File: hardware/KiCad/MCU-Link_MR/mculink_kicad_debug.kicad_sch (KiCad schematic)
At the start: 43 parts, among them J1 Pixhawk Debug Full (1x10 JST-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, J2 Pixhawk_Debug_Mini (1x06 JST-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, J6 Conn_02x05_Odd_Even, J8 DCD-LZ_Debug (1x07 JST-GHS), SW2 KMR221GLFS, U3 74LVC2T45DC, U4 SN74LVC1T45GW, U5 SN74LVC1T45GW, U6 MCP6001-OT, U7 SN74LVC1T45GW

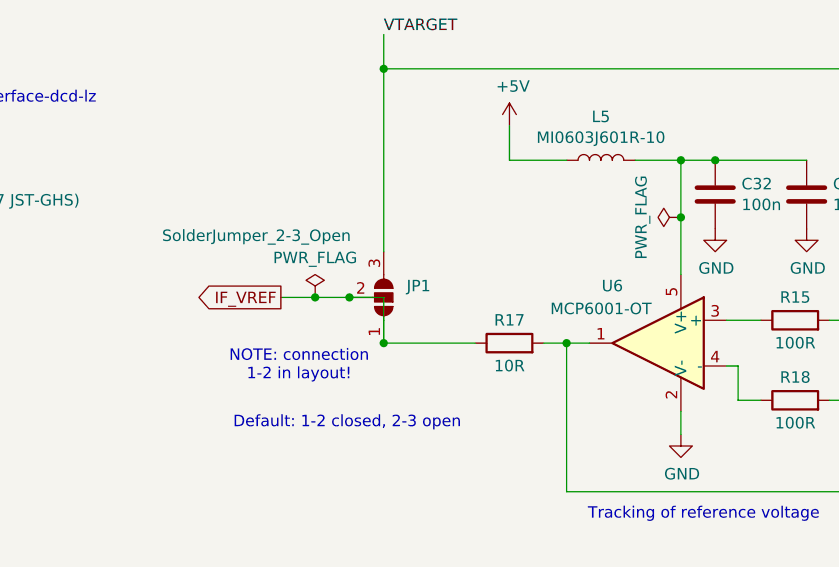
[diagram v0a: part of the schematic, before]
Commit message: cleanup
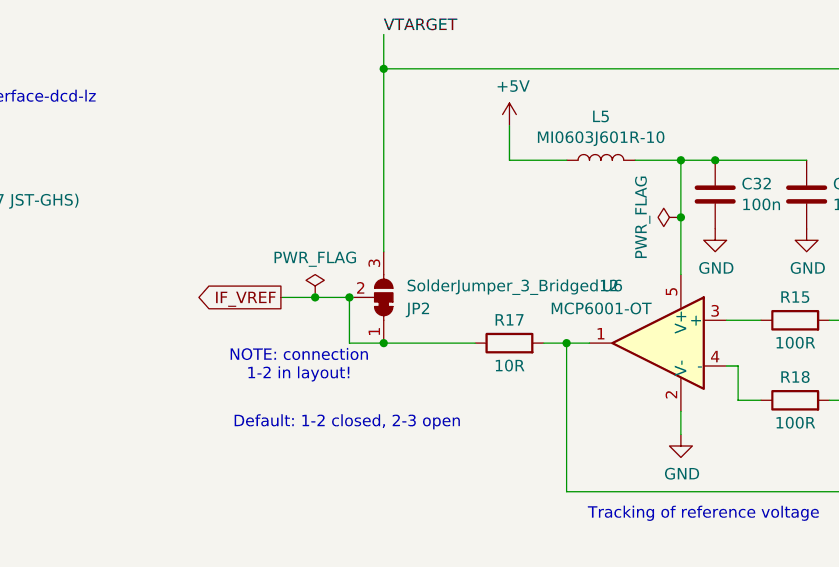
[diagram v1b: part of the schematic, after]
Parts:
- removed JP1: SolderJumper_2-3_Open, McuOnEclipse:SolderJumper-3_P1.3mm_Open_RoundedPad1.0x1.5mm, symbol Jumper:SolderJumper_3_Open
- added JP2: SolderJumper_3_Bridged12, McuOnEclipse:SolderJumper-3_P1.3mm_Open_RoundedPad1.0x1.5mm, symbol Jumper:SolderJumper_3_Bridged12
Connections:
- net IF_VREF: now also JP2.1 (A), JP2.2 (C)
- net VTARGET: now also JP2.3 (B)
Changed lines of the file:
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@@
 	)
 	(junction
-		(at 203.2 134.62)
-		(diameter 0)
-		(color 0 0 0 0)
-	)
-	(junction
 		(at 63.5 20.32)
 		(diameter 0)
@@
 	)
 	(junction
+		(at 203.2 134.62)
+		(diameter 0)
+		(color 0 0 0 0)
+	)
+	(junction
 		(at 240.03 119.38)
 		(diameter 0)
@@
 	)
 	(junction
-		(at 207.01 139.7)
-		(diameter 0)
-		(color 0 0 0 0)
-	)
-	(junction
 		(at 227.33 139.7)
 		(diameter 0)
@@
 	)
 	(junction
+		(at 207.01 139.7)
+		(diameter 0)
+		(color 0 0 0 0)
+	)
+	(junction
 		(at 33.02 20.32)
 		(diameter 0)
@@
 	(wire
 		(pts
+			(xy 203.2 134.62) (xy 203.2 139.7)
+		)
+		(stroke
+			(width 0)
+			(type default)
+		)
+	)
+	(wire
+		(pts
 			(xy 267.97 48.26) (xy 271.78 48.26)
 		)
@@
 	(wire
 		(pts
-			(xy 207.01 134.62) (xy 203.2 134.62)
-		)
-		(stroke
-			(width 0)
-			(type default)
-		)
-	)
-	(wire
-		(pts
 			(xy 257.81 156.21) (xy 227.33 156.21)
 		)
@@
 	(wire
 		(pts
-			(xy 207.01 139.7) (xy 207.01 134.62)
-		)
-		(stroke
-			(width 0)
-			(type default)
-		)
-	)
-	(wire
-		(pts
 			(xy 96.52 179.07) (xy 96.52 180.34)
 		)
@@
 	(wire
 		(pts
+			(xy 203.2 139.7) (xy 207.01 139.7)
+		)
+		(stroke
+			(width 0)
+			(type default)
+		)
+	)
+	(wire
+		(pts
 			(xy 39.37 125.73) (xy 39.37 124.46)
 		)
@@
 	)
 	(symbol
+		(lib_id "Jumper:SolderJumper_3_Bridged12")
+		(at 207.01 134.62 270)
+		(mirror x)
+		(unit 1)
+		(exclude_from_sim no)
+		(in_bom yes)
+		(on_board yes)
+		(dnp no)
+		(fields_autoplaced yes)
+		(property "Reference" "JP2"
+			(at 209.55 135.8901 90)
+			(effects
+				(font
+					(size 1.27 1.27)
+				)
+				(justify left)
+			)
+		)
+		(property "Value" "SolderJumper_3_Bridged12"
+			(at 209.55 133.3501 90)
+			(effects
+				(font
+					(size 1.27 1.27)
+				)
+				(justify left)
+			)
+		)
+		(property "Footprint" "McuOnEclipse:SolderJumper-3_P1.3mm_Open_RoundedPad1.0x1.5mm"
+			(at 207.01 134.62 0)
+			(effects
+				(font
+					(size 1.27 1.27)
+				)
+				(hide yes)
+			)
+		)
+		(property "Datasheet" "~"
+			(at 207.01 134.62 0)
+			(effects
+				(font
+					(size 1.27 1.27)
+				)
+				(hide yes)
+			)
+		)
+		(property "Description" "3-pole Solder Jumper, pins 1+2 closed/bridged"
+			(at 207.01 134.62 0)
+			(effects
+				(font
+					(size 1.27 1.27)
+				)
+				(hide yes)
+			)
+		)
+		(pin "3"
+		)
+		(pin "2"
+		)
+		(pin "1"
+		)
+		(instances
+			(project "MCU-Link_MR"
+				(path "/5d025764-753a-4b80-8d3d-c9a8a22c9527/00000000-0000-0000-0000-0000603cff19"
+					(reference "JP2")
+					(unit 1)
+				)
+			)
+		)
+	)
+	(symbol
 		(lib_id "power:GND")
 		(at 143.51 102.87 0)
@@
 					(unit 1)
 				)
-			)
-		)
-	)
-	(symbol
-		(lib_id "Jumper:SolderJumper_3_Open")
-		(at 207.01 134.62 270)
-		(mirror x)
-		(unit 1)
-		(exclude_from_sim no)
-		(in_bom yes)
-		(on_board yes)
-		(dnp no)
-		(property "Reference" "JP1"
-			(at 209.55 133.3499 90)
-			(effects
-				(font
-					(size 1.27 1.27)
-				)
-				(justify left)
-			)
-		)
-		(property "Value" "SolderJumper_2-3_Open"
-			(at 182.372 127.762 90)
-			(effects
-				(font
-					(size 1.27 1.27)
-				)
-				(justify left)
-			)
-		)
-		(property "Footprint" "McuOnEclipse:SolderJumper-3_P1.3mm_Open_RoundedPad1.0x1.5mm"
-			(at 207.01 134.62 0)
-			(effects
-				(font
-					(size 1.27 1.27)
-				)
-				(hide yes)
-			)
-		)
-		(property "Datasheet" "~"
-			(at 207.01 134.62 0)
-			(effects
-				(font
-					(size 1.27 1.27)
-				)
-				(hide yes)
-			)
-		)
-		(property "Description" "Solder Jumper, 3-pole, open"
-			(at 207.01 134.62 0)
-			(effects
-				(font
-					(size 1.27 1.27)
-				)
-				(hide yes)
-			)
-		)
-		(property "distrelec#" ""
-			(at 207.01 134.62 0)
-			(effects
-				(font
-					(size 1.27 1.27)
-				)
-				(hide yes)
-			)
-		)
-		(pin "2"
-		)
-		(pin "1"
-		)
-		(pin "3"
-		)
-		(instances
-			(project "MCU-Link_MR"
-				(path "/5d025764-753a-4b80-8d3d-c9a8a22c9527/00000000-0000-0000-0000-0000603cff19"
-					(reference "JP1")
-					(unit 1)
-				)
